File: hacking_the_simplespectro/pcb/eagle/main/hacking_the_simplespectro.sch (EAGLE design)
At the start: 56 parts, among them CON1 BAT, CON2 SPI, CON3 SPI, CON4 VIBR, IC1 32U4, IC2 MCP73831T, IC3 MCP1703CB, IC4 DMP1045U, Q6 BSP75, SW1 EC12E_SW, U1 NCT75DMR2G, X1 8MHz, X2 MINI-USB

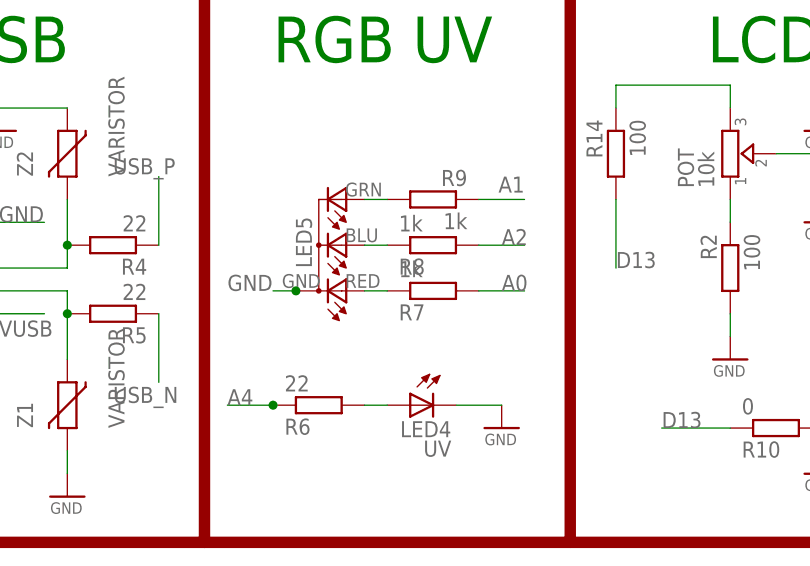
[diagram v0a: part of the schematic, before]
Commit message: update eagle
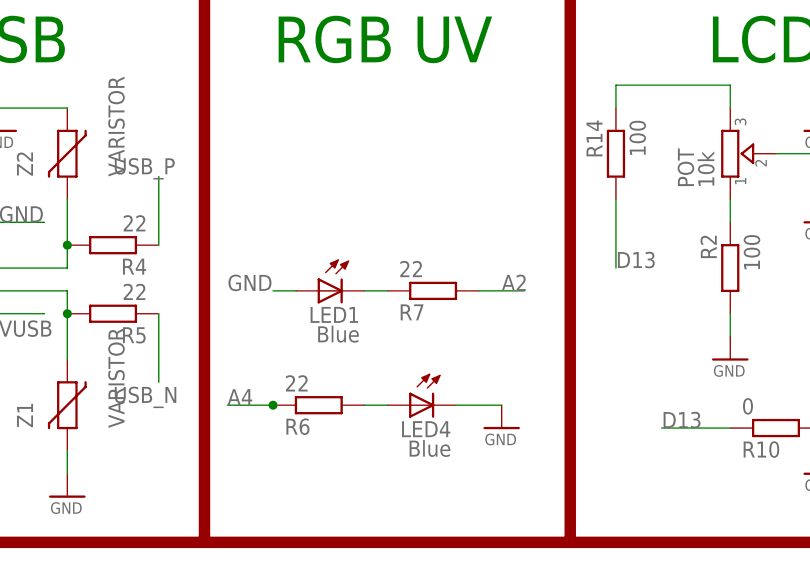
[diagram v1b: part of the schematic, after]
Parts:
- removed LED5: RGB-COMMON-CATHODE, lpatiny:RGB-COMMON-CATHODE
- removed R8, R9: 1k, rcl:R-EU_R0805
- added LED1: Blue, SparkFun:LED5MM
- LED4: value UV -> Blue
- R7: value 1k -> 22
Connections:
- removed net N$10: LED5.CBLUE, R8.1
- removed net N$9: LED5.CGREEN, R9.2
- net A0: no longer R7.2
- net A1: no longer R9.1
- net A2: now also R7.2; no longer R8.2
- net GND: now also LED1.A; no longer LED5.A2
- net N$13: now also LED1.C; no longer LED5.CRED
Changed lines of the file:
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@@
 <attribute name="LCSC" value="C17414"/>
 </part>
-<part name="R7" library="rcl" deviceset="R-EU_" device="R0805" value="1k">
+<part name="R7" library="rcl" deviceset="R-EU_" device="R0805" value="22">
 <attribute name="ELECROW" value="C17513"/>
 <attribute name="LCSC" value="C17513"/>
 </part>
-<part name="R8" library="rcl" deviceset="R-EU_" device="R0805" value="1k">
-<attribute name="ELECROW" value="C17513"/>
-<attribute name="LCSC" value="C17513"/>
-</part>
-<part name="R9" library="rcl" deviceset="R-EU_" device="R0805" value="1k">
-<attribute name="ELECROW" value="C17513"/>
-<attribute name="LCSC" value="C17513"/>
-</part>
-<part name="LED5" library="lpatiny" deviceset="RGB-COMMON-CATHODE" device=""/>
 <part name="LCD" library="HD44780LCD" deviceset="LCD-HD44780" device="16X2-4-HOLES" technology="4-HOLES"/>
 <part name="C8" library="rcl" library_urn="urn:adsk.eagle:library:334" deviceset="C-EU" device="C0805K" package3d_urn="urn:adsk.eagle:package:23681/2" value="10u">
@@
 </part>
 <part name="GND9" library="supply1" deviceset="GND" device=""/>
-<part name="LED4" library="SparkFun" deviceset="LED" device="5MM" value="UV"/>
+<part name="LED4" library="SparkFun" deviceset="LED" device="5MM" value="Blue"/>
 <part name="U$7" library="lpatiny" deviceset="TSL237" device=""/>
 <part name="U$8" library="microbuilder" deviceset="GND" device=""/>
@@
 </part>
 <part name="SW1" library="switch-alps" deviceset="EC12E_SW" device=""/>
+<part name="LED1" library="SparkFun" deviceset="LED" device="5MM" value="Blue"/>
 </parts>
 <sheets>
@@
 <attribute name="ELECROW" x="111.76" y="35.56" size="1.778" layer="96" rot="MR180" display="off"/>
 </instance>
-<instance part="R8" gate="G$1" x="111.76" y="40.64" rot="MR180">
-<attribute name="LCSC" x="111.76" y="40.64" size="1.778" layer="96" rot="MR180" display="off"/>
-<attribute name="ELECROW" x="111.76" y="40.64" size="1.778" layer="96" rot="MR180" display="off"/>
-</instance>
-<instance part="R9" gate="G$1" x="111.76" y="45.72" rot="MR0">
-<attribute name="LCSC" x="111.76" y="45.72" size="1.778" layer="96" rot="MR0" display="off"/>
-<attribute name="ELECROW" x="111.76" y="45.72" size="1.778" layer="96" rot="MR0" display="off"/>
-</instance>
-<instance part="LED5" gate="G$1" x="99.06" y="40.64" rot="R90"/>
 <instance part="LCD" gate="G$1" x="185.42" y="35.56"/>
 <instance part="C8" gate="G$1" x="-7.62" y="38.1">
@@
 <instance part="SW1" gate="G$1" x="0" y="256.54"/>
 <instance part="SW1" gate="G$2" x="22.86" y="256.54"/>
+<instance part="LED1" gate="G$1" x="99.06" y="35.56" rot="MR270"/>
 </instances>
 <busses>
@@
 </segment>
 <segment>
-<pinref part="LED5" gate="G$1" pin="A2"/>
 <wire x1="96.52" y1="35.56" x2="93.98" y2="35.56" width="0.1524" layer="91"/>
-<junction x="96.52" y="35.56"/>
 <label x="88.9" y="35.56" size="1.778" layer="95"/>
+<pinref part="LED1" gate="G$1" pin="A"/>
 </segment>
 <segment>
@@
 </segment>
 <segment>
-<pinref part="R8" gate="G$1" pin="2"/>
-<wire x1="121.92" y1="40.64" x2="116.84" y2="40.64" width="0.1524" layer="91"/>
-<label x="119.38" y="40.64" size="1.778" layer="95"/>
+<pinref part="R7" gate="G$1" pin="2"/>
+<wire x1="116.84" y1="35.56" x2="121.92" y2="35.56" width="0.1524" layer="91"/>
+<label x="119.38" y="35.56" size="1.778" layer="95"/>
 </segment>
 </net>
@@
 <label x="170.18" y="205.74" size="1.778" layer="95"/>
 </segment>
-<segment>
-<pinref part="R9" gate="G$1" pin="1"/>
-<wire x1="116.84" y1="45.72" x2="121.92" y2="45.72" width="0.1524" layer="91"/>
-<label x="121.92" y="48.26" size="1.778" layer="95" rot="R180"/>
-</segment>
 </net>
 <net name="D5" class="0">
@@
 <wire x1="160.02" y1="203.2" x2="175.26" y2="203.2" width="0.1524" layer="91"/>
 <label x="170.18" y="203.2" size="1.778" layer="95"/>
-</segment>
-<segment>
-<pinref part="R7" gate="G$1" pin="2"/>
-<wire x1="116.84" y1="35.56" x2="121.92" y2="35.56" width="0.1524" layer="91"/>
-<label x="119.38" y="35.56" size="1.778" layer="95"/>
 </segment>
 </net>
@@
 </segment>
 </net>
-<net name="N$9" class="0">
-<segment>
-<pinref part="LED5" gate="G$1" pin="CGREEN"/>
-<pinref part="R9" gate="G$1" pin="2"/>
-<wire x1="104.14" y1="45.72" x2="106.68" y2="45.72" width="0.1524" layer="91"/>
-</segment>
-</net>
-<net name="N$10" class="0">
-<segment>
-<pinref part="R8" gate="G$1" pin="1"/>
-<pinref part="LED5" gate="G$1" pin="CBLUE"/>
-<wire x1="106.68" y1="40.64" x2="104.14" y2="40.64" width="0.1524" layer="91"/>
-</segment>
-</net>
 <net name="N$13" class="0">
 <segment>
-<pinref part="LED5" gate="G$1" pin="CRED"/>
 <pinref part="R7" gate="G$1" pin="1"/>
 <wire x1="104.14" y1="35.56" x2="106.68" y2="35.56" width="0.1524" layer="91"/>
-</segment>
-</net>
+<pinref part="LED1" gate="G$1" pin="C"/>
+</segment>
+</net>
